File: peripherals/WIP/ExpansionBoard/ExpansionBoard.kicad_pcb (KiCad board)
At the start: 2 copper layers, 170.2 x 170.2 mm, 14 parts, among them J1 ExpansionPort, J2 Exp 1A, J3 Exp 1B, J4 Exp 2A, J5 Exp 2B, J6 Exp 3, J7 Exp 4, J8 Exp 5, J9 ExpansionPort, U2 AS6C4008-55PCN, U3 AS6C4008-55PCN, U5 TCA9548APWR

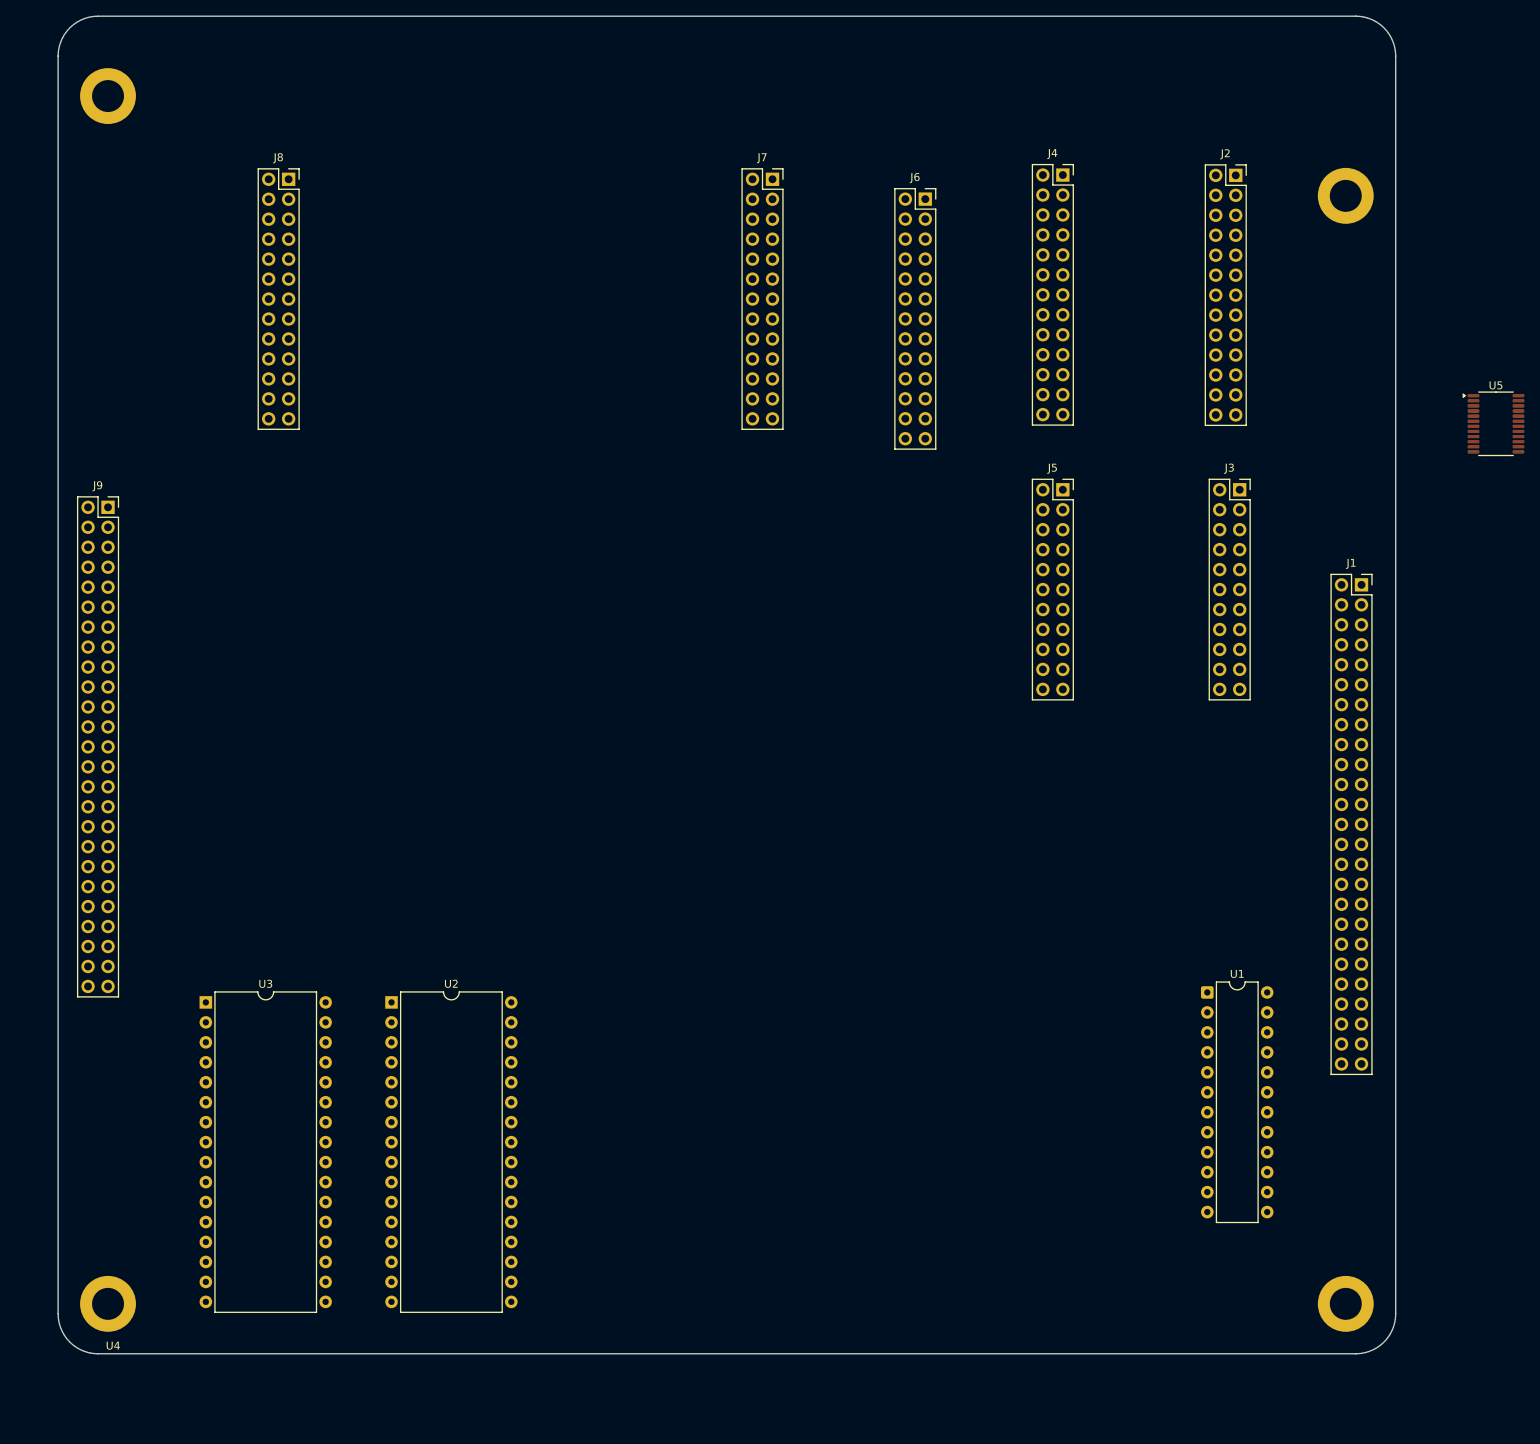
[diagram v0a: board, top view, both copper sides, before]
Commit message: Updates
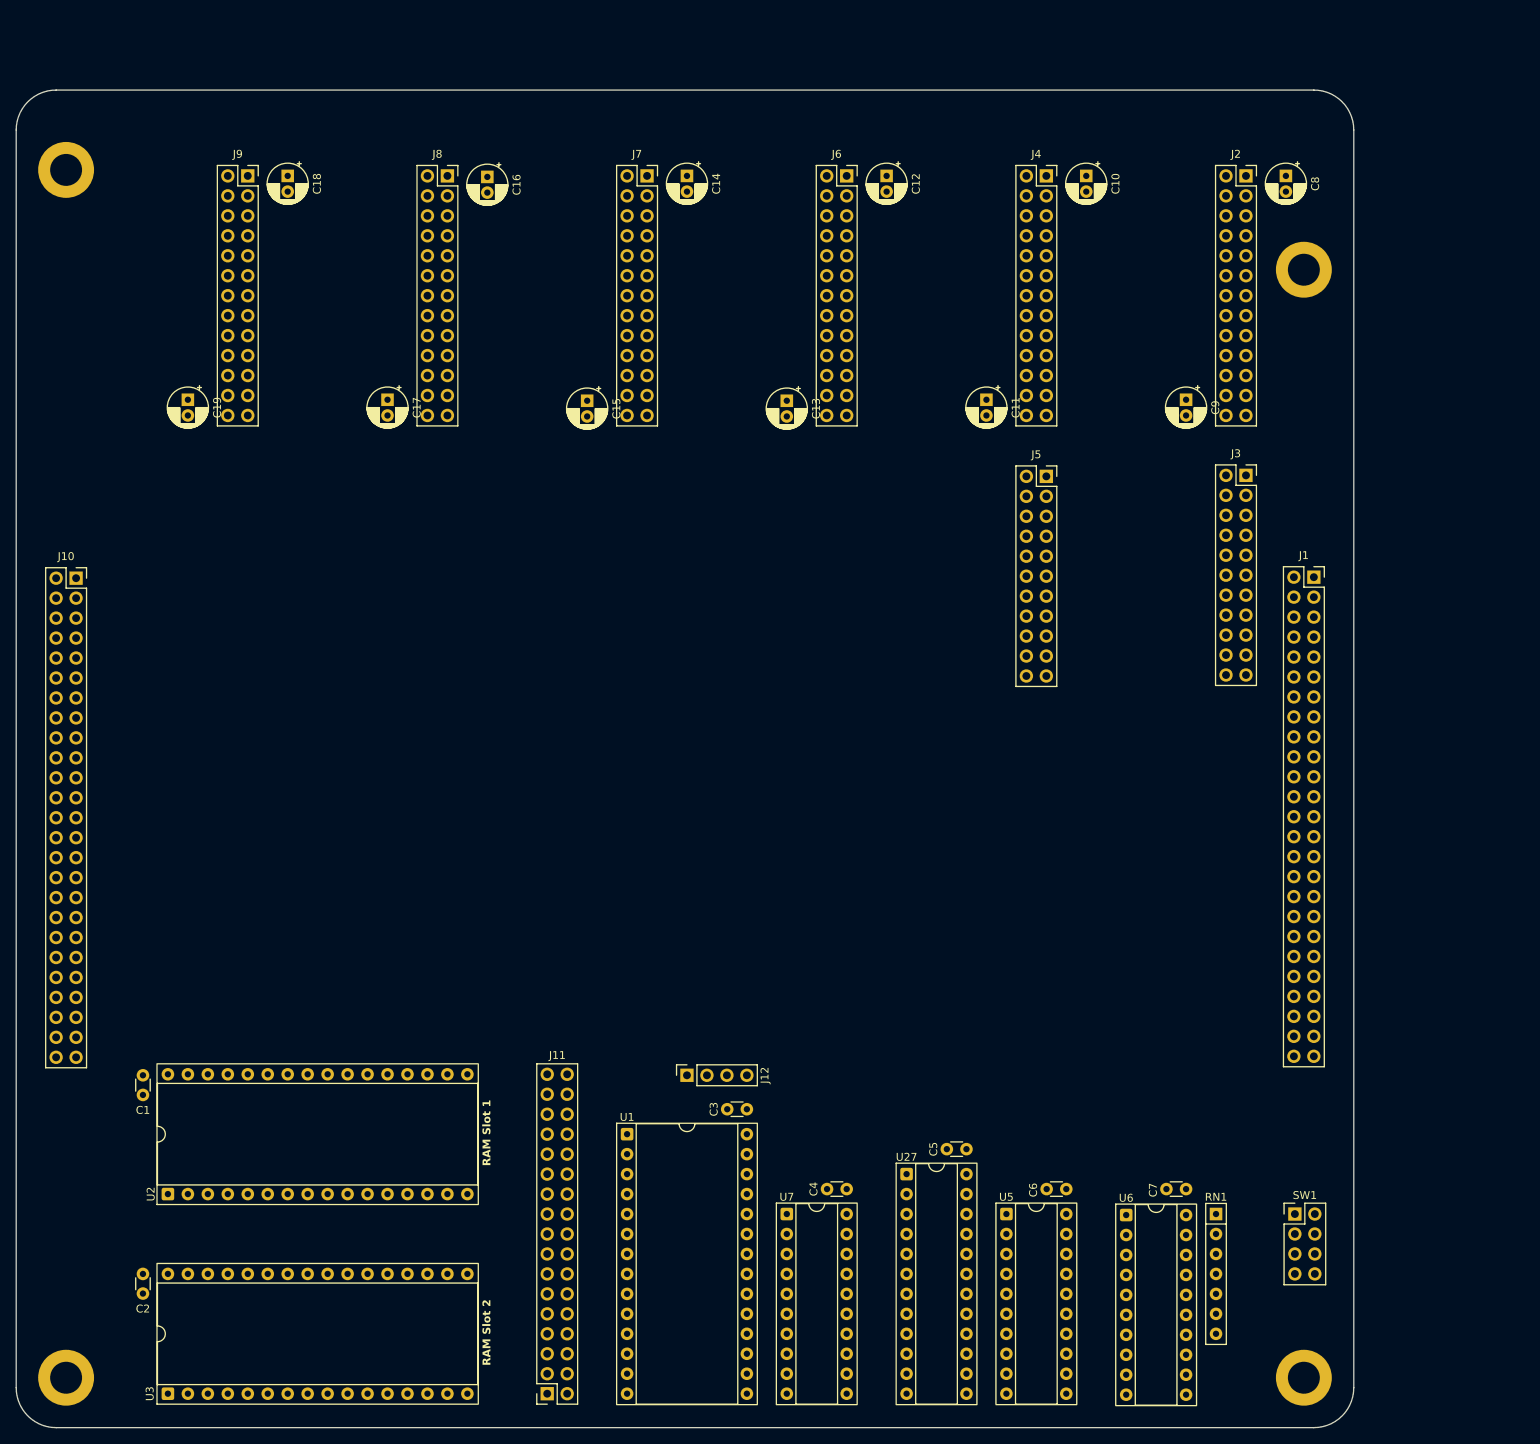
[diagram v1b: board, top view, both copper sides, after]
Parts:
- added C1: 100n, Capacitor_THT:C_Disc_D3.0mm_W1.6mm_P2.50mm, F.Cu at (37.5, 156.3)
- added C10: 10u, Capacitor_THT:CP_Radial_D5.0mm_P2.00mm, F.Cu at (157.5, 41.9)
- added C11: 10u, Capacitor_THT:CP_Radial_D5.0mm_P2.00mm, F.Cu at (144.8, 70.4)
- added C12: 10u, Capacitor_THT:CP_Radial_D5.0mm_P2.00mm, F.Cu at (132.1, 41.9)
- added C13: 10u, Capacitor_THT:CP_Radial_D5.0mm_P2.00mm, F.Cu at (119.4, 70.5)
- added C14: 10u, Capacitor_THT:CP_Radial_D5.0mm_P2.00mm, F.Cu at (106.7, 41.9)
- added C15: 10u, Capacitor_THT:CP_Radial_D5.0mm_P2.00mm, F.Cu at (94.0, 70.5)
- added C16: 10u, Capacitor_THT:CP_Radial_D5.0mm_P2.00mm, F.Cu at (81.3, 42.0)
- added C17: 10u, Capacitor_THT:CP_Radial_D5.0mm_P2.00mm, F.Cu at (68.6, 70.4)
- added C18: 10u, Capacitor_THT:CP_Radial_D5.0mm_P2.00mm, F.Cu at (55.9, 41.9)
- added C19: 10u, Capacitor_THT:CP_Radial_D5.0mm_P2.00mm, F.Cu at (43.2, 70.4)
- added C2: 100n, Capacitor_THT:C_Disc_D3.0mm_W1.6mm_P2.50mm, F.Cu at (37.5, 181.6)
- added C3: 100n, Capacitor_THT:C_Disc_D3.0mm_W1.6mm_P2.50mm, F.Cu at (114.3, 160.7)
- added C4: 100n, Capacitor_THT:C_Disc_D3.0mm_W1.6mm_P2.50mm, F.Cu at (127.0, 170.8)
- added C5: 100n, Capacitor_THT:C_Disc_D3.0mm_W1.6mm_P2.50mm, F.Cu at (142.2, 165.7)
- added C6: 100n, Capacitor_THT:C_Disc_D3.0mm_W1.6mm_P2.50mm, F.Cu at (154.9, 170.8)
- added C7: 100n, Capacitor_THT:C_Disc_D3.0mm_W1.6mm_P2.50mm, F.Cu at (170.2, 170.8)
- added C8: 10u, Capacitor_THT:CP_Radial_D5.0mm_P2.00mm, F.Cu at (182.9, 41.9)
- added C9: 10u, Capacitor_THT:CP_Radial_D5.0mm_P2.00mm, F.Cu at (170.2, 70.4)
- added J11: I2C Header, Connector_PinSocket_2.54mm:PinSocket_2x17_P2.54mm_Vertical, F.Cu at (88.9, 196.8)
- added J12: Ext. I2C, Connector_PinSocket_2.54mm:PinSocket_1x04_P2.54mm_Vertical, F.Cu at (106.7, 156.3)
- added J9: Exp 6, Connector_PinSocket_2.54mm:PinSocket_2x13_P2.54mm_Vertical, F.Cu at (50.8, 41.9)
- added RN1: 10k, Resistor_THT:R_Array_SIP7, F.Cu at (174.0, 174.0)
- added SW1: SW_DIP_x04, Connector_PinHeader_2.54mm:PinHeader_2x04_P2.54mm_Vertical, F.Cu at (184.0, 174.0)
- added U27: GAL 22V10, Package_DIP:DIP-24_W7.62mm_Socket, F.Cu at (134.6, 168.9)
- added U6: 74LS245, Package_DIP:DIP-20_W7.62mm_Socket, F.Cu at (162.6, 174.1)
- added U7: 74LS540, Package_DIP:DIP-20_W7.62mm_Socket, F.Cu at (119.4, 174.0)
- U1: value ~ -> 8259A; footprint Package_DIP:DIP-24_W7.62mm -> Package_DIP:DIP-28_W15.24mm_Socket
- U2, U3: footprint Package_DIP:DIP-32_W15.24mm -> Package_DIP:DIP-32_W15.24mm_Socket
- U4: value ~ -> Motherboard Outline
- U5: value TCA9548APWR -> GAL16V8; footprint Package_SO:TSSOP-24_4.4x7.8mm_P0.65mm -> Package_DIP:DIP-20_W7.62mm_Socket
- moved U5 118.3 mm to (147.3, 174.0)
- moved U1 76.0 mm to (99.1, 163.8)
- moved U3 50.0 mm to (40.6, 196.8), turned to 90 degrees
- moved U2 37.5 mm to (40.6, 171.4), turned to 90 degrees
- moved J8 20.2 mm to (76.2, 41.9)
- moved J7 16.0 mm to (101.6, 41.9)
- moved U4 10.8 mm to (21.3, 201.2)
- moved J6 10.4 mm to (127.0, 41.9)
- moved J10 9.89 mm to (29.0, 93.1)
- moved J1 6.14 mm to (186.4, 93.0)
- moved J5 2.70 mm to (152.4, 80.1)
- moved J4 2.10 mm to (152.4, 41.9)
- moved J3 2.00 mm to (177.8, 80.0)
- moved J2 1.30 mm to (177.8, 41.9)
- renumbered J9 to J10
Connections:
- net R/_W renamed R/~{W}
- net _BREQ renamed ~{BREQ}
- net _EN_E1 renamed ~{EN_E1}
- net _EN_E2 renamed ~{EN_E2}
- net _EN_E3 renamed ~{EN_E3}
- net _EN_E4 renamed ~{EN_E4}
- net _EN_E5 renamed ~{EN_E5}
- net _MAP_EN renamed ~{MAP_EN}
- J1 pad 15: /~{WR} -> ~{WR}
- J1 pad 25: /~{RD} -> ~{RD}
- J1 pad 42: A14 -> /A14
- J1 pad 44: A15 -> /A15
- J1 pad 45: unconnected-(J1-Pin_45-Pad45) -> /AM20
- J1 pad 46: AM21 -> /AM21
- J1 pad 5: E -> /E
- J1 pad 7: BAVAIL -> /BAVAIL
- J1 pad 8: AM20 -> +12V
- J1 pad 9: AM19 -> /AM19
- J10 pad 15: /~{WR} -> ~{WR}
- J10 pad 25: /~{RD} -> ~{RD}
- J10 pad 42: A14 -> /A14
- J10 pad 44: A15 -> /A15
- J10 pad 45: unconnected-(J9-Pin_45-Pad45) -> /AM20
- J10 pad 46: AM21 -> /AM21
- J10 pad 5: E -> /E
- J10 pad 7: BAVAIL -> /BAVAIL
- J10 pad 8: AM20 -> +12V
- J10 pad 9: AM19 -> /AM19
- J2 pad 10: _WR -> ~{WR}
- J2 pad 2: _RST -> ~{RST}
- J2 pad 23: unconnected-(J2-Pin_23-Pad23) -> SCL1
- J2 pad 25: unconnected-(J2-Pin_25-Pad25) -> SDA1
- J2 pad 4: _IRQ_E1 -> ~{IRQ_E1}
- J2 pad 8: _RD -> ~{RD}
- J4 pad 10: _WR -> ~{WR}
- J4 pad 2: _RST -> ~{RST}
- J4 pad 23: unconnected-(J4-Pin_23-Pad23) -> SCL2
- J4 pad 25: GND -> SDA2
- J4 pad 4: _IRQ_E2 -> ~{IRQ_E2}
- J4 pad 8: _RD -> ~{RD}
- J6 pad 10: _WR -> ~{WR}
- J6 pad 2: _RST -> ~{RST}
- J6 pad 23: unconnected-(J6-Pin_23-Pad23) -> SCL3
- J6 pad 25: GND -> SDA3
- J6 pad 4: _IRQ_E3 -> ~{IRQ_E3}
- J6 pad 8: _RD -> ~{RD}
- J7 pad 10: _WR -> ~{WR}
- J7 pad 2: _RST -> ~{RST}
- J7 pad 23: unconnected-(J7-Pin_23-Pad23) -> SCL4
- J7 pad 25: GND -> SDA4
- J7 pad 4: _IRQ_E4 -> ~{IRQ_E4}
- J7 pad 8: _RD -> ~{RD}
- J8 pad 10: _WR -> ~{WR}
- J8 pad 2: _RST -> ~{RST}
- J8 pad 23: unconnected-(J8-Pin_23-Pad23) -> SCL5
- J8 pad 25: GND -> SDA5
- J8 pad 4: _IRQ_E5 -> ~{IRQ_E5}
- J8 pad 8: _RD -> ~{RD}
- U1 pad 1: unconnected-(U1-I1/CLK-Pad1) -> ~{IRQ_EN}
- U1 pad 10: unconnected-(U1-I10-Pad10) -> D1
- U1 pad 11: unconnected-(U1-I11-Pad11) -> D0
- U1 pad 14: unconnected-(U1-I10-Pad14) -> GND
- U1 pad 17: unconnected-(U1-IO7-Pad17) -> EXP_IRQ
- U1 pad 18: unconnected-(U1-IO6-Pad18) -> Net-(U1-IR0)
- U1 pad 19: unconnected-(U1-IO5-Pad19) -> Net-(U1-IR1)
- U1 pad 2: unconnected-(U1-I2-Pad2) -> ~{WR}
- U1 pad 20: unconnected-(U1-IO4-Pad20) -> Net-(U1-IR2)
- U1 pad 21: unconnected-(U1-I03-Pad21) -> Net-(U1-IR3)
- U1 pad 22: unconnected-(U1-IO2-Pad22) -> Net-(U1-IR4)
- U1 pad 23: unconnected-(U1-IO1-Pad23) -> Net-(U1-IR5)
- U1 pad 24: unconnected-(U1-VCC-Pad24) -> Net-(U1-IR6)
- U1 pad 3: unconnected-(U1-I3-Pad3) -> ~{RD}
- U1 pad 4: unconnected-(U1-I4-Pad4) -> D7
- U1 pad 5: unconnected-(U1-I5-Pad5) -> D6
- U1 pad 6: unconnected-(U1-I6-Pad6) -> D5
- U1 pad 7: unconnected-(U1-I7-Pad7) -> D4
- U1 pad 8: unconnected-(U1-I8-Pad8) -> D3
- U1 pad 9: unconnected-(U1-I9-Pad9) -> D2
- U2 pad 1: unconnected-(U2-A18-Pad1) -> AM18
- U2 pad 10: unconnected-(U2-A2-Pad10) -> A2
- U2 pad 11: unconnected-(U2-A1-Pad11) -> A1
- U2 pad 12: unconnected-(U2-A0-Pad12) -> A0
- U2 pad 13: unconnected-(U2-DQ0-Pad13) -> D0
- U2 pad 14: unconnected-(U2-DQ1-Pad14) -> D1
- U2 pad 15: unconnected-(U2-DQ2-Pad15) -> D2
- U2 pad 16: unconnected-(U2-VSS-Pad16) -> GND
- U2 pad 17: unconnected-(U2-DQ3-Pad17) -> D3
- U2 pad 18: unconnected-(U2-DQ4-Pad18) -> D4
- U2 pad 19: unconnected-(U2-DQ5-Pad19) -> D5
- U2 pad 2: unconnected-(U2-A16-Pad2) -> AM16
- U2 pad 20: unconnected-(U2-DQ6-Pad20) -> D6
- U2 pad 21: unconnected-(U2-DQ7-Pad21) -> D7
- U2 pad 22: unconnected-(U2-CE#-Pad22) -> ~{RAMX_L_EN}
- U2 pad 23: unconnected-(U2-A10-Pad23) -> A10
- U2 pad 24: unconnected-(U2-OE#-Pad24) -> ~{RD}
- U2 pad 25: unconnected-(U2-A11-Pad25) -> A11
- U2 pad 26: unconnected-(U2-A9-Pad26) -> A9
- U2 pad 27: unconnected-(U2-A8-Pad27) -> A8
- U2 pad 28: unconnected-(U2-A13-Pad28) -> A13
- U2 pad 29: unconnected-(U2-WE#-Pad29) -> ~{WR}
- U2 pad 3: unconnected-(U2-A14-Pad3) -> AM14
- U2 pad 30: unconnected-(U2-A17-Pad30) -> AM17
- U2 pad 31: unconnected-(U2-A15-Pad31) -> AM15
- U2 pad 32: unconnected-(U2-VCC-Pad32) -> VCC
- U2 pad 4: unconnected-(U2-A12-Pad4) -> A12
- U2 pad 5: unconnected-(U2-A7-Pad5) -> A7
- U2 pad 6: unconnected-(U2-A6-Pad6) -> A6
- U2 pad 7: unconnected-(U2-A5-Pad7) -> A5
- U2 pad 8: unconnected-(U2-A4-Pad8) -> A4
- U2 pad 9: unconnected-(U2-A3-Pad9) -> A3
- U3 pad 1: unconnected-(U3-A18-Pad1) -> AM18
- U3 pad 10: unconnected-(U3-A2-Pad10) -> A2
- U3 pad 11: unconnected-(U3-A1-Pad11) -> A1
- U3 pad 12: unconnected-(U3-A0-Pad12) -> A0
- U3 pad 13: unconnected-(U3-DQ0-Pad13) -> D0
- U3 pad 14: unconnected-(U3-DQ1-Pad14) -> D1
- U3 pad 15: unconnected-(U3-DQ2-Pad15) -> D2
- U3 pad 16: unconnected-(U3-VSS-Pad16) -> GND
- U3 pad 17: unconnected-(U3-DQ3-Pad17) -> D3
- U3 pad 18: unconnected-(U3-DQ4-Pad18) -> D4
- U3 pad 19: unconnected-(U3-DQ5-Pad19) -> D5
- U3 pad 2: unconnected-(U3-A16-Pad2) -> AM16
- U3 pad 20: unconnected-(U3-DQ6-Pad20) -> D6
- U3 pad 21: unconnected-(U3-DQ7-Pad21) -> D7
- U3 pad 22: unconnected-(U3-CE#-Pad22) -> ~{RAMX_H_EN}
- U3 pad 23: unconnected-(U3-A10-Pad23) -> A10
- U3 pad 24: unconnected-(U3-OE#-Pad24) -> ~{RD}
- U3 pad 25: unconnected-(U3-A11-Pad25) -> A11
- U3 pad 26: unconnected-(U3-A9-Pad26) -> A9
- U3 pad 27: unconnected-(U3-A8-Pad27) -> A8
- U3 pad 28: unconnected-(U3-A13-Pad28) -> A13
- U3 pad 29: unconnected-(U3-WE#-Pad29) -> ~{WR}
- U3 pad 3: unconnected-(U3-A14-Pad3) -> AM14
- U3 pad 30: unconnected-(U3-A17-Pad30) -> AM17
- U3 pad 31: unconnected-(U3-A15-Pad31) -> AM15
- U3 pad 32: unconnected-(U3-VCC-Pad32) -> VCC
- U3 pad 4: unconnected-(U3-A12-Pad4) -> A12
- U3 pad 5: unconnected-(U3-A7-Pad5) -> A7
- U3 pad 6: unconnected-(U3-A6-Pad6) -> A6
- U3 pad 7: unconnected-(U3-A5-Pad7) -> A5
- U3 pad 8: unconnected-(U3-A4-Pad8) -> A4
- U3 pad 9: unconnected-(U3-A3-Pad9) -> A3
- U5 pad 1: GND -> /~{EXP_EN}
- U5 pad 10: unconnected-(U5-SD3-Pad10) -> GND
- U5 pad 11: unconnected-(U5-SC3-Pad11) -> BOARD_SEL
- U5 pad 12: GND -> EXP_IRQ
- U5 pad 13: unconnected-(U5-SD4-Pad13) -> /~{EX_IRQ}
- U5 pad 17: unconnected-(U5-SD6-Pad17) -> ~{I2C_EN}
- U5 pad 18: unconnected-(U5-SC6-Pad18) -> ~{IRQ_EN}
- U5 pad 19: unconnected-(U5-SD7-Pad19) -> ~{INFO_EN}
- U5 pad 2: GND -> A0
- U5 pad 20: unconnected-(U5-SC7-Pad20) -> VCC
- U5 pad 3: _RST -> A1
- U5 pad 4: unconnected-(U5-SD0-Pad4) -> A2
- U5 pad 5: unconnected-(U5-SC0-Pad5) -> A3
- U5 pad 6: unconnected-(U5-SD1-Pad6) -> A4
- U5 pad 7: unconnected-(U5-SC1-Pad7) -> A5
- U5 pad 8: unconnected-(U5-SD2-Pad8) -> A6
- U5 pad 9: unconnected-(U5-SC2-Pad9) -> A8
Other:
- board text added: "RAM Slot 1"
- board text added: "RAM Slot 2"
